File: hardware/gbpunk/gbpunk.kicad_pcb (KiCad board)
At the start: 2 copper layers, 57.5 x 82 mm, 64 parts, among them J1 CART, J2 SWD_CONNECTOR, J4 SWD_CONNECTOR, P1 USB_C_CONNECTOR, SW7 RESET, SW9 USB_BOOT, U1 RP2040, U2 SN74LVC4245A, U3 W25Q128JVS, U4 NCP1117-3.3_SOT223, U5 SN74LVC4245A, U6 SN74LVC4245A, U7 SN74LVC4245A, Y1 12MHz

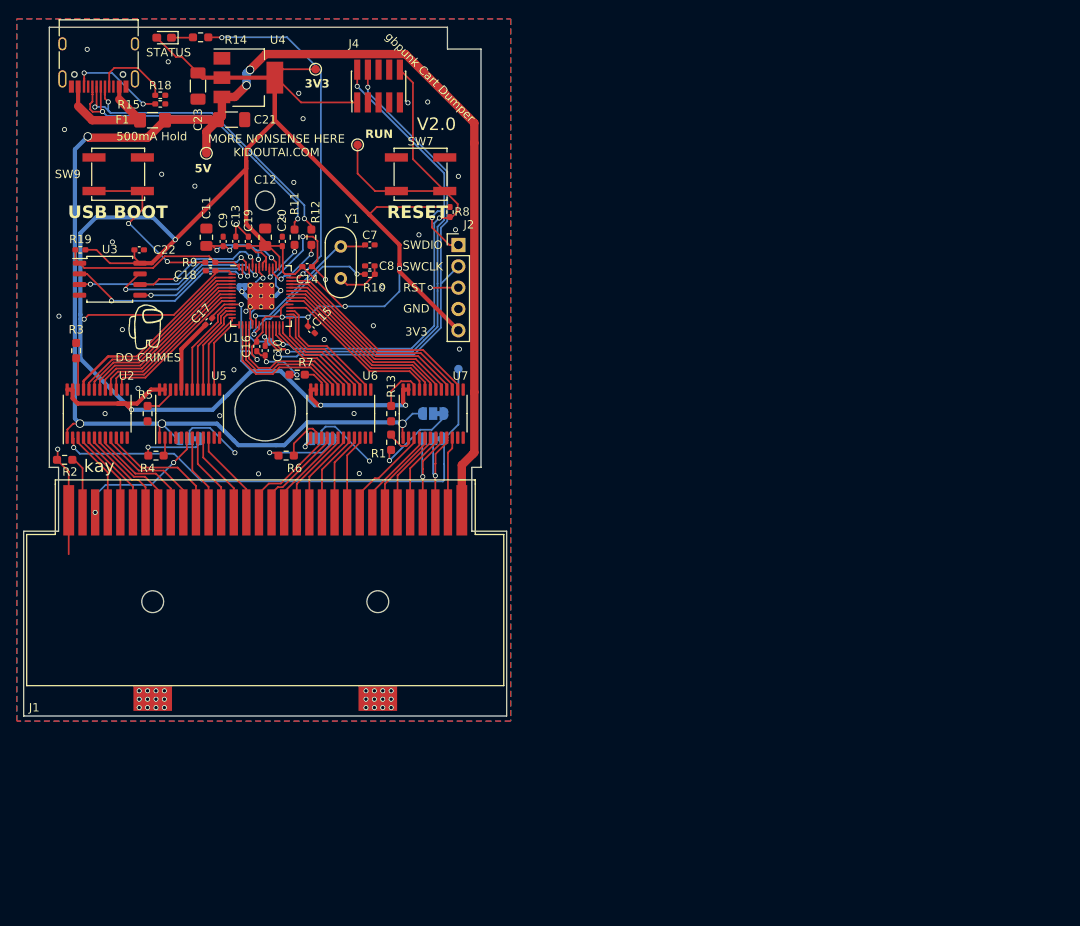
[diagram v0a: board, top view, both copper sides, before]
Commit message: need to double check but hardware rev looks good
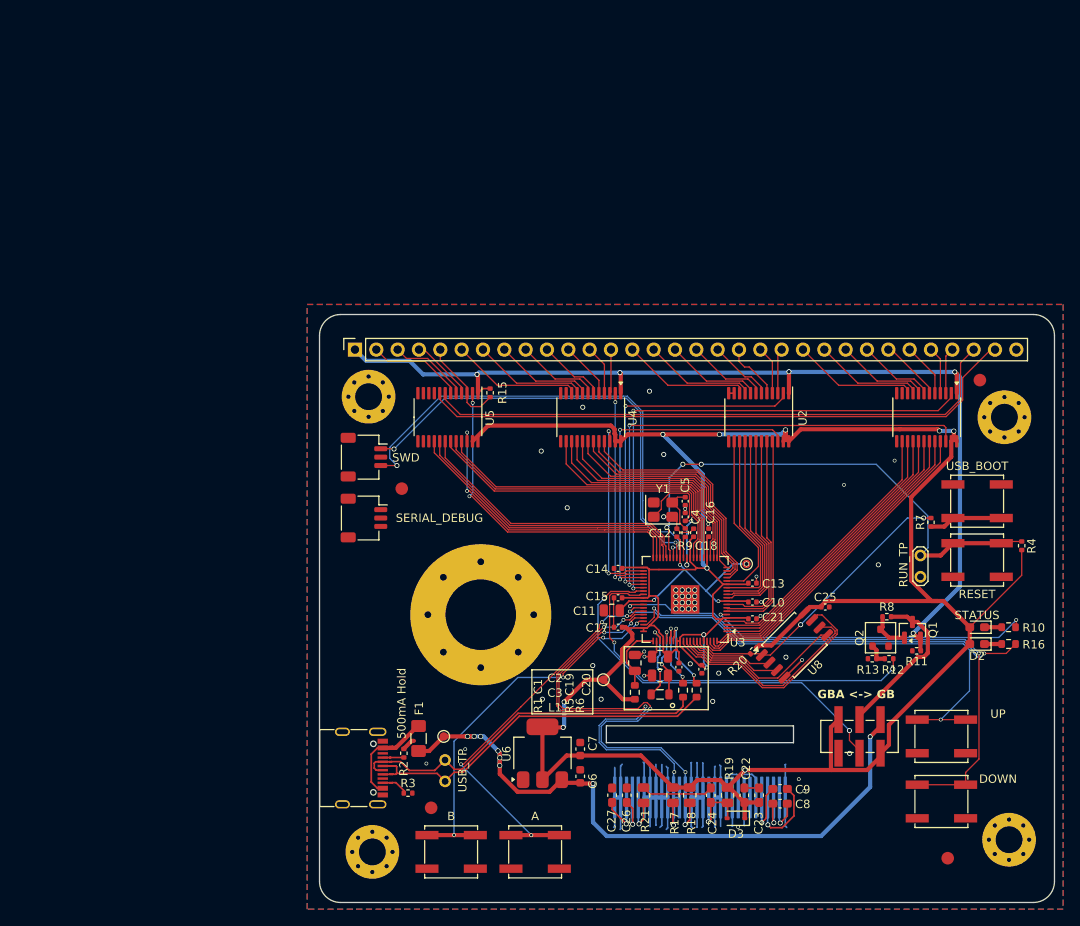
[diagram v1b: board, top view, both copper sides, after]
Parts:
- removed G***: LOGO, gbpunk:sussy
- removed G***: LOGO, gbpunk:cart
- removed G***: LOGO, gbpunk:logo
- removed JP1, JP3, JP4: SWDIR_1, Jumper:SolderJumper-3_P1.3mm_Bridged12_RoundedPad1.0x1.5mm
- removed JP2: SWDIR_0, Jumper:SolderJumper-3_P1.3mm_Bridged12_RoundedPad1.0x1.5mm
- removed MK1: DNF, Gekkio_MountingHole:MountingHole_7.2mm
- removed MK2: DNF, Gekkio_MountingHole:MountingHole_2.3mm
- removed P1: USB_C_CONNECTOR, Connector_USB:USB_C_Receptacle_HRO_TYPE-C-31-M-12
- removed R14: 330, Resistor_SMD:R_0603_1608Metric_Pad0.98x0.95mm_HandSolder
- removed SW9: USB_BOOT, Button_Switch_SMD:SW_SPST_EVPBF
- added C1: 4.7uF, Capacitor_SMD:C_0805_2012Metric, F.Cu at (144.0, 114.7)
- added C2: 4.7uF, Capacitor_SMD:C_0805_2012Metric, F.Cu at (147.0, 113.9)
- added C24: 10uF, Capacitor_SMD:C_0603_1608Metric_Pad1.08x0.95mm_HandSolder, F.Cu at (153.1, 130.4)
- added C25: 100nF, Capacitor_SMD:C_0402_1005Metric, F.Cu at (166.7, 108.0)
- added C26: 10uF, Capacitor_SMD:C_0603_1608Metric_Pad1.08x0.95mm_HandSolder, F.Cu at (143.1, 130.4)
- added C27: 10uF, Capacitor_SMD:C_0603_1608Metric_Pad1.08x0.95mm_HandSolder, F.Cu at (141.3, 130.4)
- added C3: 4.7uF, Capacitor_SMD:C_0805_2012Metric, F.Cu at (147.0, 116.2)
- added C4: 15p, Capacitor_SMD:C_0402_1005Metric, F.Cu at (150.0, 97.3)
- added C5: 15p, Capacitor_SMD:C_0402_1005Metric, F.Cu at (150.0, 95.4)
- added C6: 10uF, Capacitor_SMD:C_0603_1608Metric, F.Cu at (137.5, 128.2)
- added D2: ERR, LED_SMD:LED_0603_1608Metric_Pad1.05x0.95mm_HandSolder, F.Cu at (184.8, 112.4)
- added D3: 1N4148WS, Diode_SMD:D_SOD-323, F.Cu at (156.1, 133.2)
- added FID1: Fiducial, Fiducial:Fiducial_1.5mm_Mask3mm, F.Cu at (119.8, 131.9)
- added FID2: Fiducial, Fiducial:Fiducial_1.5mm_Mask3mm, F.Cu at (116.3, 93.9)
- added FID3: Fiducial, Fiducial:Fiducial_1.5mm_Mask3mm, F.Cu at (185.1, 81.0)
- added FID4: Fiducial, Fiducial:Fiducial_1.5mm_Mask3mm, F.Cu at (181.3, 137.9)
- added H1: MOUNT, MountingHole:MountingHole_3.2mm_M3_Pad_Via, F.Cu at (112.3, 83.0)
- added H2: MOUNT, MountingHole:MountingHole_3.2mm_M3_Pad_Via, F.Cu at (188.6, 135.7)
- added H3: MOUNT, MountingHole:MountingHole_3.2mm_M3_Pad_Via, F.Cu at (112.8, 137.2)
- added H4: MOUNT, MountingHole:MountingHole_3.2mm_M3_Pad_Via, F.Cu at (188.0, 85.4)
- added H5: TRIPOD, MountingHole:MountingHole_8.4mm_M8_Pad_Via, F.Cu at (125.7, 108.9)
- added J3: USB, Connector_USB:USB_C_Receptacle_G-Switch_GT-USB-7010ASV, F.Cu at (110.3, 127.2)
- added L1: 3.3uH, Inductor_SMD:L_0805_2012Metric, F.Cu at (147.0, 118.4)
- added Q1: AO3401A, Package_TO_SOT_SMD:SOT-23, F.Cu at (177.1, 110.7)
- added Q2: 2N7002, PCM_Package_TO_SOT_SMD_AKL:SOT-23, F.Cu at (173.3, 111.7)
- added R16: 330, Resistor_SMD:R_0603_1608Metric, F.Cu at (188.5, 112.4)
- added R17: 4.7k, Resistor_SMD:R_0805_2012Metric, F.Cu at (148.6, 130.4)
- added R20: 10k, Resistor_SMD:R_0402_1005Metric, F.Cu at (158.1, 113.2)
- added R21: 390k, Resistor_SMD:R_0805_2012Metric, F.Cu at (145.1, 130.4)
- added SW1: RESET, Button_Switch_SMD:SW_SPST_EVPBF, F.Cu at (184.8, 102.4)
- added SW2: USB_BOOT, Button_Switch_SMD:SW_SPST_EVPBF, F.Cu at (184.8, 95.4)
- added SW3: DOWN, Button_Switch_SMD:SW_SPST_EVPBF, F.Cu at (180.5, 131.2)
- added SW4: UP, Button_Switch_SMD:SW_SPST_EVPBF, F.Cu at (180.5, 123.4)
- added SW5: CART_TYPE_SELECT, gbpunk:SW_DPDT_CK_JS202011JCQN, F.Cu at (170.8, 123.4)
- added SW6: A, Button_Switch_SMD:SW_SPST_EVPBF, F.Cu at (132.1, 137.2)
- added U8: W25Q128JVS, Package_SO:SOIC-8_5.3x5.3mm_P1.27mm, F.Cu at (163.0, 112.6)
- C10, C13, C14, C15, C16, C17, C18, C19, C20: footprint Capacitor_SMD:C_0402_1005Metric_Pad0.74x0.62mm_HandSolder -> Capacitor_SMD:C_0402_1005Metric
- C11: value 1uF -> 4.7uF; footprint Capacitor_SMD:C_0805_2012Metric_Pad1.18x1.45mm_HandSolder -> Capacitor_SMD:C_0805_2012Metric
- C12: value 1uF -> 100nF; footprint Capacitor_SMD:C_0805_2012Metric_Pad1.18x1.45mm_HandSolder -> Capacitor_SMD:C_0402_1005Metric
- C21: value 10uF -> 100nF; footprint Capacitor_SMD:C_1206_3216Metric_Pad1.33x1.80mm_HandSolder -> Capacitor_SMD:C_0402_1005Metric
- C22: value 100nF -> 10uF; footprint Capacitor_SMD:C_0402_1005Metric_Pad0.74x0.62mm_HandSolder -> Capacitor_SMD:C_0603_1608Metric_Pad1.08x0.95mm_HandSolder
- C23: footprint Capacitor_SMD:C_1206_3216Metric_Pad1.33x1.80mm_HandSolder -> Capacitor_SMD:C_0603_1608Metric_Pad1.08x0.95mm_HandSolder
- C7: value 27pF -> 10uF; footprint Capacitor_SMD:C_0402_1005Metric_Pad0.74x0.62mm_HandSolder -> Capacitor_SMD:C_0603_1608Metric
- C8: value 27pF -> 2.2uF; footprint Capacitor_SMD:C_0402_1005Metric_Pad0.74x0.62mm_HandSolder -> Capacitor_SMD:C_0603_1608Metric_Pad1.08x0.95mm_HandSolder
- C9: value 100nF -> 2.2uF; footprint Capacitor_SMD:C_0402_1005Metric_Pad0.74x0.62mm_HandSolder -> Capacitor_SMD:C_0603_1608Metric_Pad1.08x0.95mm_HandSolder
- J1: value CART -> SERIAL_DEBUG; footprint gbpunk:gbpunk_aliexpress_gb_connector -> Connector_JST:JST_SH_SM03B-SRSS-TB_1x03-1MP_P1.00mm_Horizontal
- J2: value SWD_CONNECTOR -> SWD; footprint Connector_PinHeader_2.54mm:PinHeader_1x05_P2.54mm_Vertical -> Connector_JST:JST_SH_SM03B-SRSS-TB_1x03-1MP_P1.00mm_Horizontal
- J4: value SWD_CONNECTOR -> CART; footprint Connector_PinHeader_1.27mm:PinHeader_2x05_P1.27mm_Vertical_SMD -> Connector_PinSocket_2.54mm:PinSocket_1x32_P2.54mm_Vertical
- R1: value 1k -> 33; footprint Resistor_SMD:R_0603_1608Metric_Pad0.98x0.95mm_HandSolder -> Resistor_SMD:R_0603_1608Metric
- R10: value 1k -> 330; footprint Resistor_SMD:R_0402_1005Metric_Pad0.72x0.64mm_HandSolder -> Resistor_SMD:R_0603_1608Metric
- R11: value 27 -> 10k; footprint Resistor_SMD:R_0603_1608Metric_Pad0.98x0.95mm_HandSolder -> Resistor_SMD:R_0402_1005Metric
- R12: value 27 -> 270; footprint Resistor_SMD:R_0603_1608Metric_Pad0.98x0.95mm_HandSolder -> Resistor_SMD:R_0402_1005Metric
- R13, R4: value 1k -> 10k; footprint Resistor_SMD:R_0603_1608Metric_Pad0.98x0.95mm_HandSolder -> Resistor_SMD:R_0402_1005Metric
- R15: value 56k -> 1k; footprint Resistor_SMD:R_0402_1005Metric_Pad0.72x0.64mm_HandSolder -> Resistor_SMD:R_0402_1005Metric
- R18: value 56k -> 4.7k; footprint Resistor_SMD:R_0402_1005Metric_Pad0.72x0.64mm_HandSolder -> Resistor_SMD:R_0805_2012Metric
- R19: value 10k -> 4.7k; footprint Resistor_SMD:R_0402_1005Metric_Pad0.72x0.64mm_HandSolder -> Resistor_SMD:R_0805_2012Metric
- R2, R3: value 1k -> 5.1k; footprint Resistor_SMD:R_0603_1608Metric_Pad0.98x0.95mm_HandSolder -> Resistor_SMD:R_0402_1005Metric
- R5, R6: value 1k -> 27; footprint Resistor_SMD:R_0603_1608Metric_Pad0.98x0.95mm_HandSolder -> Resistor_SMD:R_0603_1608Metric
- R7: footprint Resistor_SMD:R_0603_1608Metric_Pad0.98x0.95mm_HandSolder -> Resistor_SMD:R_0402_1005Metric
- R8, R9: footprint Resistor_SMD:R_0402_1005Metric_Pad0.72x0.64mm_HandSolder -> Resistor_SMD:R_0402_1005Metric
- SW7: value RESET -> B
- TP1: moved to F.Cu
- TP2: value RUN_TP -> 3V3_TP
- TP3: value 3V3_TP -> RUN_TP; footprint TestPoint:TestPoint_Pad_D1.0mm -> TestPoint:TestPoint_2Pads_Pitch2.54mm_Drill0.8mm
- TP4: value DBUS_DIR_TP -> USB_TP; footprint TestPoint:TestPoint_Pad_D1.0mm -> TestPoint:TestPoint_2Pads_Pitch2.54mm_Drill0.8mm
- TP5: value 5V0_TP -> VBUS_TP
- U1: value RP2040 -> SN74LVC4245A; footprint gbpunk:RP2040-QFN-56 -> Package_SO:TSSOP-24_4.4x7.8mm_P0.65mm
- U3: value W25Q128JVS -> RP2350B; footprint Package_SO:SOIC-8_5.23x5.23mm_P1.27mm -> Package_DFN_QFN:QFN-80-1EP_10x10mm_P0.4mm_EP3.4x3.4mm
- U4: value NCP1117-3.3_SOT223 -> SN74LVC4245A; footprint Package_TO_SOT_SMD:SOT-223-3_TabPin2 -> Package_SO:TSSOP-24_4.4x7.8mm_P0.65mm
- U6: value SN74LVC4245A -> NCP1117-3.3_SOT223; footprint Package_SO:TSSOP-24_4.4x7.8mm_P0.65mm -> Package_TO_SOT_SMD:SOT-223-3_TabPin2
- U7: value SN74LVC4245A -> SSD1306; footprint Package_SO:TSSOP-24_4.4x7.8mm_P0.65mm -> gbpunk:SSD1306; moved to B.Cu
- Y1: footprint Crystal:Crystal_HC52-8mm_Vertical -> Crystal:Crystal_SMD_3225-4Pin_3.2x2.5mm
- moved D1 119.6 mm to (184.8, 110.4)
- moved C23 107.7 mm to (158.8, 130.4), turned to 90 degrees
- moved R18 104.5 mm to (150.6, 130.4), turned to 90 degrees
- moved R4 103.6 mm to (190.1, 100.7), turned to 90 degrees
- moved R19 100.8 mm to (155.1, 130.4), turned to -90 degrees
- moved C22 97.0 mm to (157.1, 130.4), turned to 90 degrees
- moved TP3 94.0 mm to (178.0, 104.4), turned to 90 degrees
- moved C9 93.0 mm to (161.3, 129.7), turned to 180 degrees
- moved R11 88.9 mm to (177.6, 113.2), turned to 0 degrees
- moved R10 86.9 mm to (188.5, 110.4), turned to 0 degrees
- moved C21 85.9 mm to (158.0, 109.4)
- moved R12 85.1 mm to (174.3, 114.2), turned to 0 degrees
- moved SW7 80.8 mm to (122.1, 137.2), turned to 180 degrees
- moved U1 80.6 mm to (178.8, 85.4), turned to -90 degrees
- moved C8 80.5 mm to (161.3, 131.4)
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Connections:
- C12 pad 1: +3.3V -> +1V1
- C21 pad 1: +5V -> +3.3V
- C7 pad 1: Net-(C7-Pad1) -> +3.3V
- C8 pad 1: Net-(C8-Pad1) -> Net-(U7-C2P)
- C8 pad 2: GND -> Net-(U7-C2N)
- C9 pad 1: +1V1 -> Net-(U7-C1P)
- C9 pad 2: GND -> Net-(U7-C1N)
- D1 pad 1: Net-(D1-Pad1) -> Net-(D1-K)
- F1 pad 1: +5V -> VBUS
- F1 pad 2: VBUS -> Net-(F1-Pad2)
- J1 pad 1: +5V -> /DEBUG_RX
- J1 pad 2: /CLK -> GND
- J1 pad 3: /~{WR} -> /DEBUG_TX
- J2 pad 1: /SWDIO -> /SWCLK
- J2 pad 2: /SWCLK -> GND
- J2 pad 3: /RUN -> /SWDIO
- J4 pad 1: +3.3V -> /GB_POWER_SW
- J4 pad 10: /RUN -> /A4
- J4 pad 2: /SWDIO -> /CLK
- J4 pad 3: GND -> /~{WR}
- J4 pad 4: /SWCLK -> /~{RD}
- J4 pad 5: GND -> /~{CS}
- J4 pad 6: unconnected-(J4-Pad6) -> /A0
- J4 pad 7: unconnected-(J4-Pad7) -> /A1
- J4 pad 8: unconnected-(J4-Pad8) -> /A2
- J4 pad 9: GND -> /A3
- R1 pad 1: Net-(R1-Pad1) -> +3.3V
- R1 pad 2: Net-(JP2-Pad1) -> /VREG_AVDD
- R10 pad 1: Net-(C8-Pad1) -> Net-(D1-K)
- R10 pad 2: Net-(R10-Pad2) -> Net-(U3-GPIO8)
- R11 pad 1: /USB_DP -> GND
- R11 pad 2: Net-(R11-Pad2) -> /GB_POWER_SW
- R12 pad 1: /USB_DM -> Net-(Q2-G)
- R12 pad 2: Net-(R12-Pad2) -> /GB_POWER_EN
- R13 pad 1: Net-(R13-Pad1) -> GND
- R13 pad 2: GND -> Net-(Q2-G)
- R15 pad 1: unconnected-(R15-Pad1) -> /GB_POWER_SW
- R15 pad 2: GND -> /~{CS}
- R18 pad 1: Net-(P1-PadA5) -> /SCREEN_SCL
- R18 pad 2: GND -> +3.3V
- R19 pad 2: /~{QSPI_CS} -> Net-(D3-A)
- R2 pad 1: Net-(J1-Pad31) -> GND
- R2 pad 2: GND -> Net-(J3-CC1)
- R3 pad 1: Net-(R3-Pad1) -> Net-(J3-CC2)
- R4 pad 1: Net-(R4-Pad1) -> +3.3V
- R4 pad 2: Net-(JP3-Pad1) -> Net-(SW1-B)
- R5 pad 1: Net-(R5-Pad1) -> /USB_DM
- R5 pad 2: GND -> Net-(U3-USB_DM)
- R6 pad 1: Net-(R6-Pad1) -> /USB_DP
- R6 pad 2: Net-(JP4-Pad1) -> Net-(U3-USB_DP)
- R7 pad 1: Net-(R7-Pad1) -> /~{QSPI_CS}
- R7 pad 2: GND -> /~{USB_BOOT}
- R8 pad 1: +3.3V -> Net-(Q1-G)
- R8 pad 2: /RUN -> Net-(Q1-D)
- R9 pad 1: /~{QSPI_CS} -> Net-(C5-Pad2)
- R9 pad 2: /~{USB_BOOT} -> Net-(U3-XOUT)
- SW7 pad 2: /RUN -> /B
- TP2 pad 1: /RUN -> +3.3V
- TP3 pad 1: +3.3V -> GND
- TP4 pad 1: Net-(JP1-Pad1) -> /USB_DP
- TP5 pad 1: +5V -> VBUS
- U1 pad 1: +3.3V -> /GB_POWER_SW
- U1 pad 10: +3.3V -> /D0
- U1 pad 11: /RST_L -> GND
- U1 pad 12: /A15_L -> GND
- U1 pad 13: /A14_L -> GND
- U1 pad 14: /A13_L -> /D0_L
- U1 pad 15: /A12_L -> /D1_L
- U1 pad 16: /A11_L -> /D2_L
- U1 pad 17: /A10_L -> /D3_L
- U1 pad 18: /A9_L -> /D4_L
- U1 pad 19: GND -> /D5_L
- U1 pad 2: /D7_L -> /DBUS_DIR
- U1 pad 20: Net-(C7-Pad1) -> /D6_L
- U1 pad 21: Net-(R10-Pad2) -> /D7_L
- U1 pad 22: +3.3V -> /DBUS_OE
- U1 pad 23: +1V1 -> +3.3V
- U1 pad 24: /SWCLK -> +3.3V
- U1 pad 3: /D6_L -> /D7
- U1 pad 4: /D5_L -> /D6
- U1 pad 5: /D4_L -> /D5
- U1 pad 6: /D3_L -> /D4
- U1 pad 7: /D2_L -> /D3
- U1 pad 8: /D1_L -> /D2
- U1 pad 9: /D0_L -> /D1
- U2 pad 1: +5V -> /GB_POWER_SW
- U2 pad 10: /D0 -> /A8
- U2 pad 14: /D0_L -> /A8_L
- U2 pad 15: /D1_L -> /A9_L
- U2 pad 16: /D2_L -> /A10_L
- U2 pad 17: /D3_L -> /A11_L
- U2 pad 18: /D4_L -> /A12_L
- U2 pad 19: /D5_L -> /A13_L
- U2 pad 2: Net-(JP1-Pad1) -> /ABUS1_DIR
- U2 pad 20: /D6_L -> /A14_L
- U2 pad 21: /D7_L -> /A15_L
- U2 pad 22: Net-(R3-Pad1) -> /ABUS1_OE
- U2 pad 3: /D7 -> /A15
- U2 pad 4: /D6 -> /A14
- U2 pad 5: /D5 -> /A13
- U2 pad 6: /D4 -> /A12
- U2 pad 7: /D3 -> /A11
- U2 pad 8: /D2 -> /A10
- U2 pad 9: /D1 -> /A9
- U3 pad 1: /~{QSPI_CS} -> /D3_L
- U3 pad 2: /QSPI_D1 -> /D2_L
- U3 pad 3: /QSPI_D2 -> /D1_L
- U3 pad 4: GND -> /D0_L
- U3 pad 5: /QSPI_D0 -> +3.3V
- U3 pad 6: /QSPI_CLK -> Net-(U3-GPIO8)
- U3 pad 7: /QSPI_D3 -> /A15_L
- U3 pad 8: +3.3V -> /A14_L
- U4 pad 1: GND -> /GB_POWER_SW
- U4 pad 2: +3.3V -> /ABUS0_DIR
- U4 pad 3: +5V -> /A7
- U5 pad 1: +5V -> /GB_POWER_SW
- U5 pad 10: /A12 -> GND
- U5 pad 14: /A12_L -> GND
- U5 pad 15: /A13_L -> GND
- U5 pad 16: /A14_L -> /IRQ_L
- U5 pad 17: /A15_L -> /RST_L
- U5 pad 18: /RST_L -> /CLK_L
- U5 pad 19: GND -> /~{WR_L}
- U5 pad 2: Net-(R4-Pad1) -> /CTLBUS_DIR
- U5 pad 20: GND -> /~{RD_L}
- U5 pad 21: GND -> /~{CS_L}
- U5 pad 22: Net-(R5-Pad1) -> /CTLBUS_OE
- U5 pad 3: GND -> /~{CS}
- U5 pad 4: GND -> /~{RD}
- U5 pad 5: GND -> /~{WR}
- U5 pad 6: /RST -> /CLK
- U5 pad 7: /A15 -> /RST
- U5 pad 8: /A14 -> /IRQ
- U5 pad 9: /A13 -> GND
- U6 pad 1: +5V -> GND
- U6 pad 2: Net-(R6-Pad1) -> +3.3V
- U6 pad 3: /A11 -> VBUS
- U7 pad 1: +5V -> GND
- U7 pad 10: /CLK -> GND
- U7 pad 11: GND -> +3.3V
- U7 pad 14: /CLK_L -> Net-(D3-A)
- U7 pad 15: /~{WR_L} -> GND
- U7 pad 16: /~{RD_L} -> GND
- U7 pad 17: /~{CS_L} -> GND
- U7 pad 18: /A0_L -> /SCREEN_SCL
- U7 pad 19: /A1_L -> /SCREEN_SDA
- U7 pad 2: Net-(R1-Pad1) -> Net-(U7-C2P)
- U7 pad 20: /A2_L -> /SCREEN_SDA
- U7 pad 21: /A3_L -> GND
- U7 pad 22: Net-(R13-Pad1) -> GND
- U7 pad 23: +3.3V -> GND
- U7 pad 24: +3.3V -> GND
- U7 pad 3: /A3 -> Net-(U7-C2N)
- U7 pad 4: /A2 -> Net-(U7-C1P)
- U7 pad 5: /A1 -> Net-(U7-C1N)
- U7 pad 6: /A0 -> +3.3V
- U7 pad 7: /~{CS} -> unconnected-(U7-NC-Pad7)
- U7 pad 8: /~{RD} -> GND
- U7 pad 9: /~{WR} -> +3.3V
- Y1 pad 1: Net-(C8-Pad1) -> Net-(U3-XIN)
- Y1 pad 2: Net-(C7-Pad1) -> GND
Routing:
- net +5V: track 199.4 -> 0.00 mm, vias 7 -> 0
- net /GB_POWER_SW: track 0.00 -> 121.5 mm, vias 0 -> 5
- net /RUN: track 75.7 -> 0.00 mm, vias 3 -> 0
- net /IRQ: track 0.00 -> 72.6 mm
- net /DOWN: track 0.00 -> 67.8 mm, vias 0 -> 2
- net VBUS: track 15.4 -> 79.5 mm, vias 0 -> 8
- net Net-(SW1-B): track 0.00 -> 61.6 mm, vias 0 -> 3
- net /DBUS_DIR: track 0.00 -> 61.4 mm, vias 0 -> 2
- net Net-(JP1-Pad1): track 61.0 -> 0.00 mm, vias 1 -> 0
- net /DBUS_OE: track 0.00 -> 60.1 mm, vias 0 -> 2
- net /UP: track 0.00 -> 59.6 mm, vias 0 -> 2
- net /SCREEN_SCL: track 0.00 -> 57.6 mm, vias 0 -> 5
- net /SCREEN_SDA: track 0.00 -> 57.6 mm, vias 0 -> 5
- net /RST: track 16.6 -> 70.1 mm, vias 2 -> 0
- net Net-(U3-GPIO47/ADC7): track 0.00 -> 49.0 mm, vias 0 -> 2
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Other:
- board size 57.5 x 82 mm -> 87.5 x 70 mm
- board text added: "GBA <-> GB"
- board text removed: "1V1"
- board text removed: "3V3"
- board text removed: "5V"
- board text removed: "A message to all aspiring engineers: Don't worry. I don't know what I'm doing either"
- board text removed: "DO CRIMES"
- board text removed: "GND"
- board text removed: "HACK THE PLANET"
- board text removed: "I don't wanna go to work I just wanna learn about esoteric gameboy mappers"
- board text removed: "MORE NONSENSE HERE KIDOUTAI.COM"
- board text removed: "PCB size: 51.4x61mm PCB thickness: 1.0mm"
- board text removed: "RESET"
- board text removed: "RST"
- board text removed: "RUN"
- board text removed: "SWCLK"
- board text removed: "SWDIO"
- board text removed: "USB BOOT"
- board text removed: "V2.0"
- board text removed: "Works Cited: github.com/Gekkio mgba-emu.github.io/gbdoc gbdev.gg8.se"
- board text removed: "You wage wars, murder, cheat, lie to us and try to make us believe it's for our own good, yet we're the criminals. Yes, I am a criminal. My crime is that of curiosity."
- board text removed: "gbpunk Cart Dumper"
- board text removed: "kay"
